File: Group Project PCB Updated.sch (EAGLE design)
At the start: 12 parts, among them J2 1X04_SMD_STRAIGHT_COMBO, J3 1x3 RA Female .1", J4 1X04_SMD_STRAIGHT_COMBO, J5 1X04_SMD_STRAIGHT_COMBO, J7 1X04_SMD_STRAIGHT_COMBO, J8 1x3 RA Female .1"

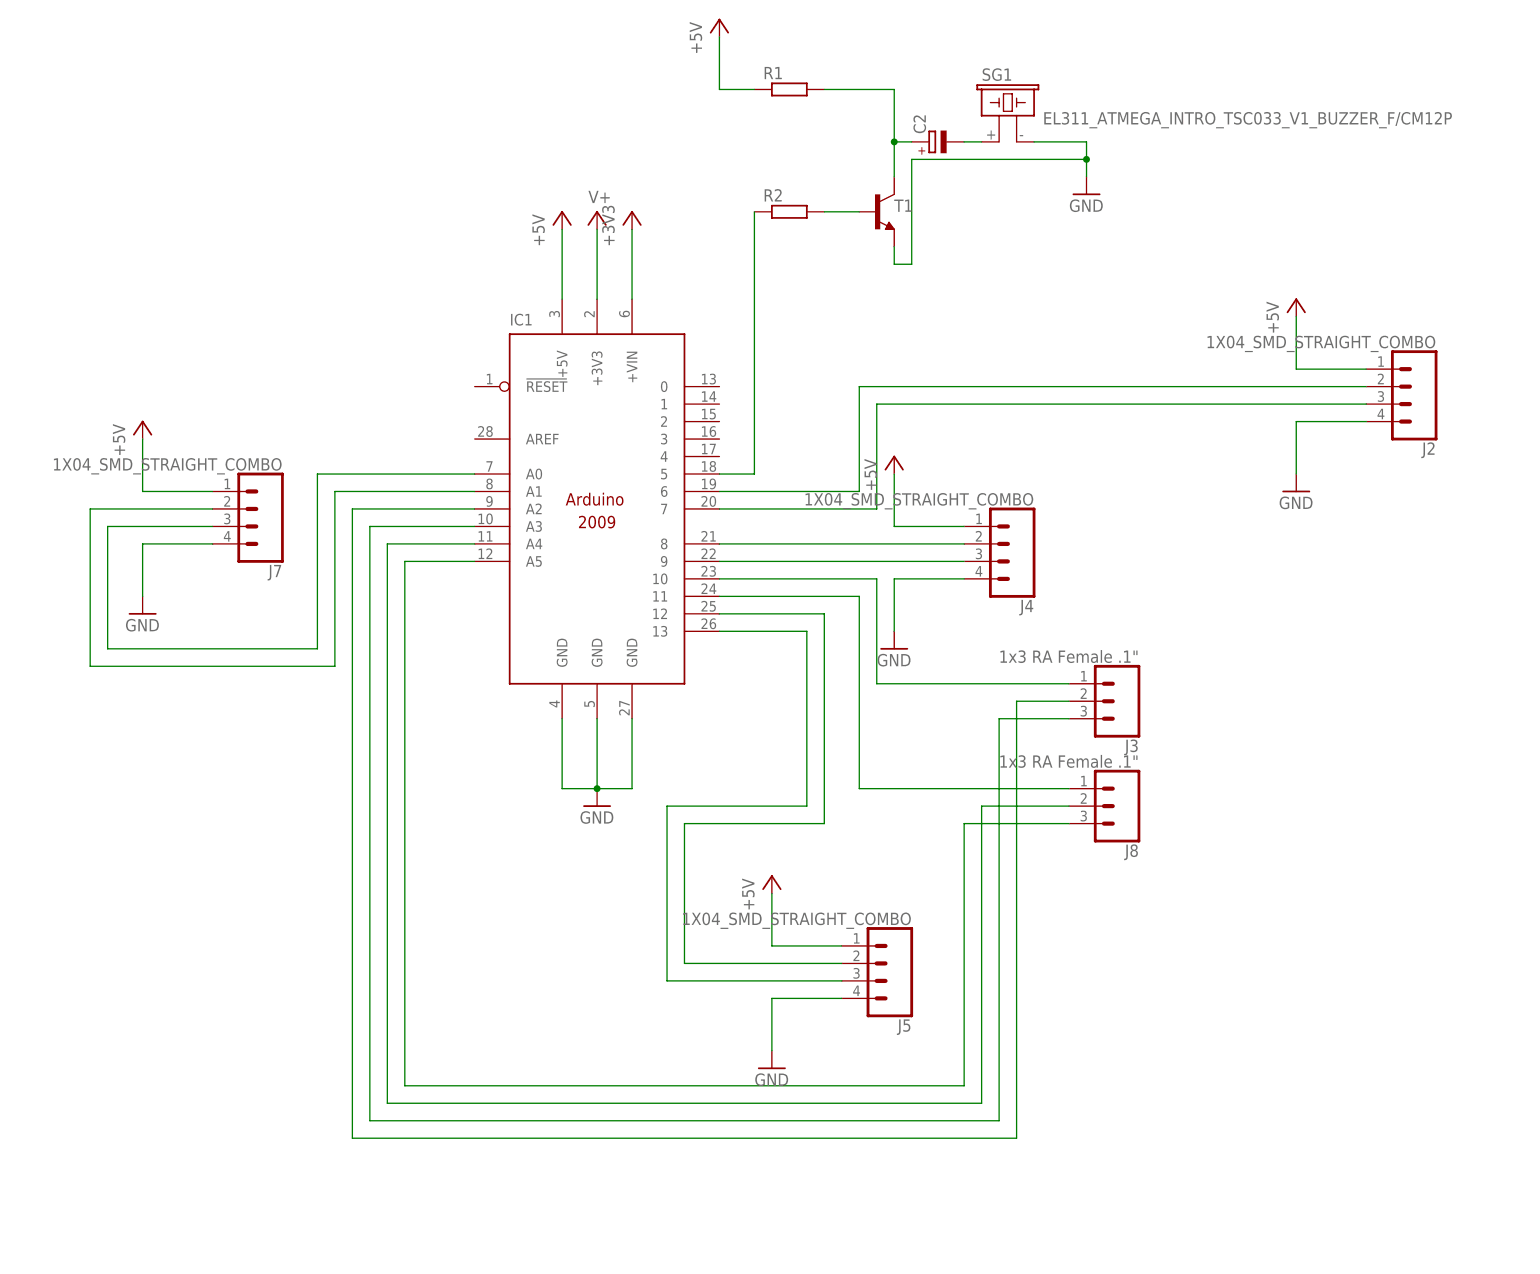
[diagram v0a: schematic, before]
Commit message: Add files via upload
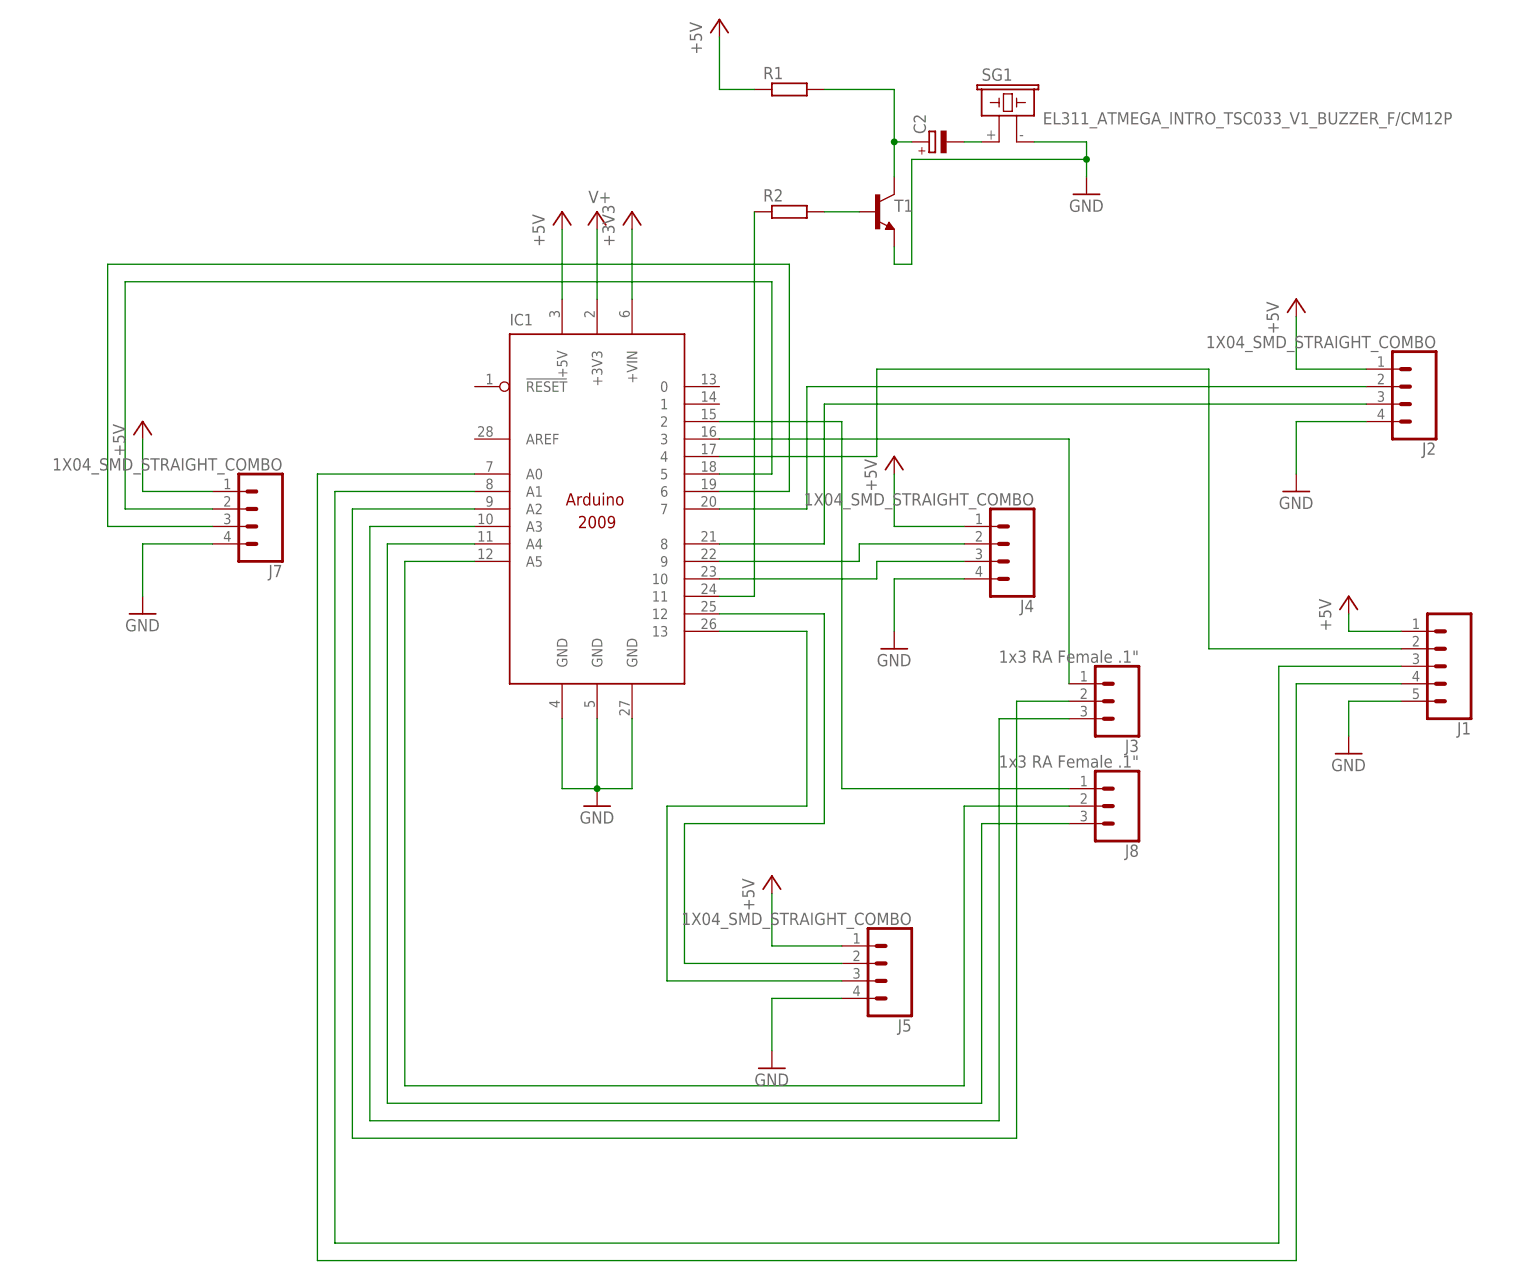
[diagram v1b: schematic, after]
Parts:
- added J1: (no value), EENG3110 V1 Library:CONN_05PTH_LONGPADS
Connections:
- new net N$19: IC1.A0, J1.4
- new net N$20: IC1.A1, J1.3
- new net N$21: IC1.4, J1.2
- net +5V: now also J1.1
- net GND: now also J1.5
- net N$12: now also IC1.2, J8.1; no longer IC1.5, R2.1
- net N$13: now also IC1.3; no longer IC1.10
- net N$14: now also R2.1; no longer J8.1
- net N$16: now also J8.3; no longer J8.2
- net N$18: now also J8.2; no longer J8.3
- net N$3: now also IC1.10, J4.3; no longer IC1.8, J4.2
- net N$4: now also J4.2; no longer J4.3
- net N$5: now also IC1.8, J2.3; no longer IC1.6, J2.2
- net N$6: now also J2.2; no longer J2.3
- net N$7: now also IC1.6, J7.3; no longer IC1.A1, J7.2
- net N$8: now also IC1.5, J7.2; no longer IC1.A0, J7.3
